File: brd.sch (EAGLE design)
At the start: 15 parts, among them IC1 OP27Z, X1 BNC-H, X2 BNC-H, X3 BNC-H, X4 BNC-H

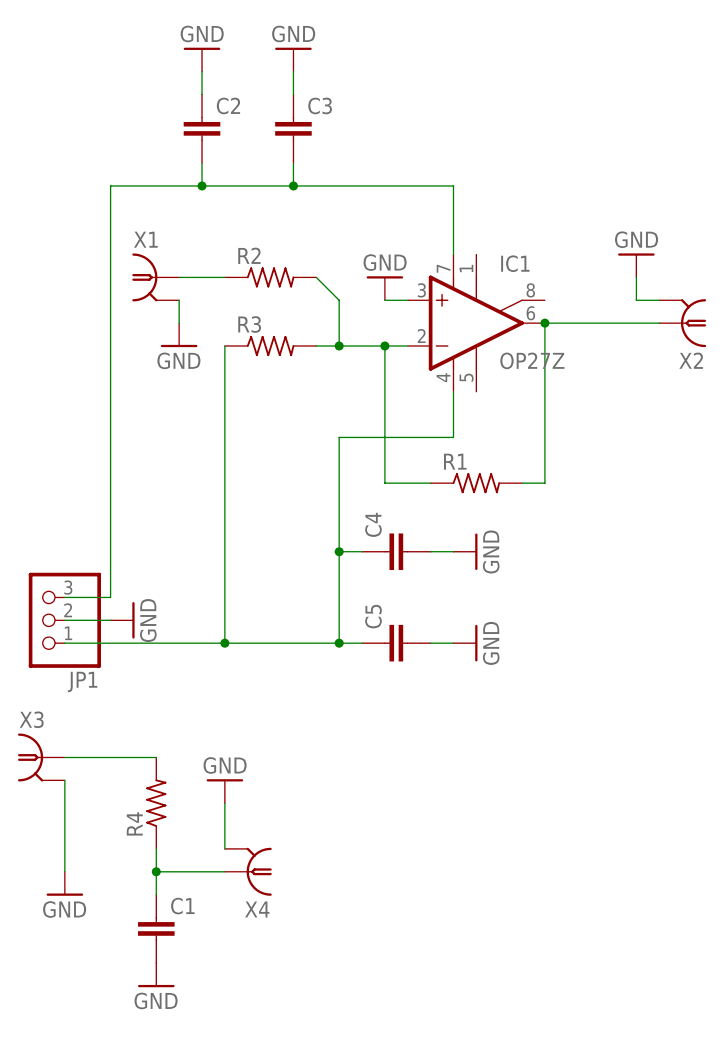
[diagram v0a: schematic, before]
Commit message: better circuit
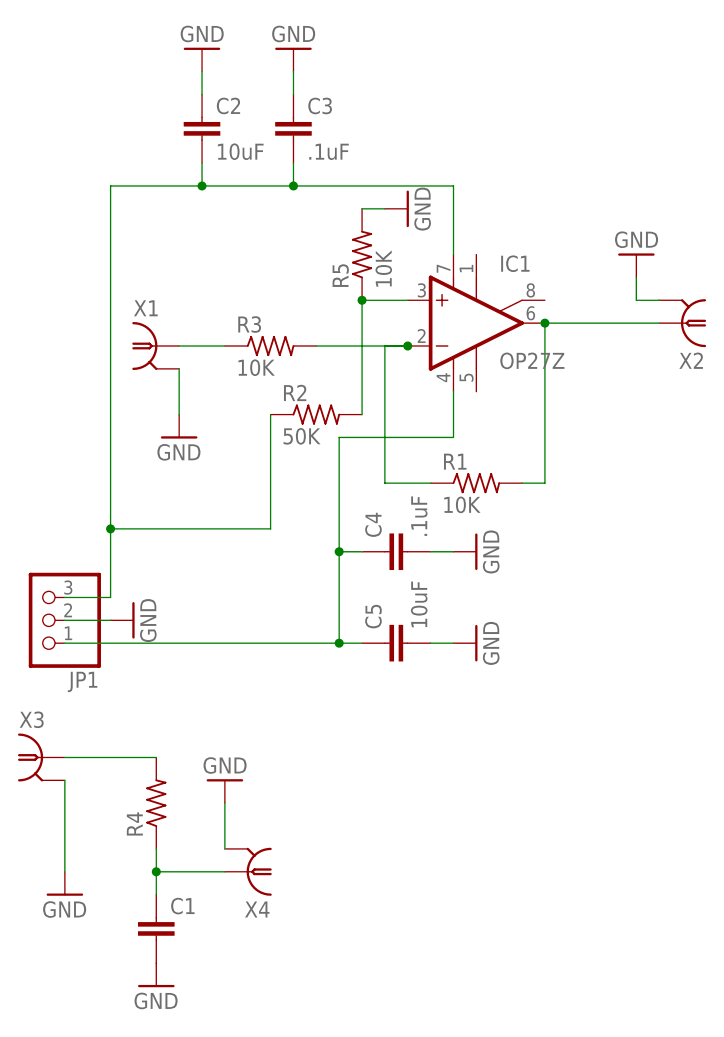
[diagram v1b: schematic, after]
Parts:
- added R5: 10K, resistor:R-US_0204/2V
- C2, C5: value (none) -> 10uF
- C3, C4: value (none) -> .1uF
- R1, R3: value (none) -> 10K
- R2: value (none) -> 50K
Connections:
- new net N$9: IC1.+IN, R2.2, R5.1
- net GND: now also R5.2; no longer IC1.+IN
- net N$1: no longer R2.2
- net N$3: no longer R3.1
- net N$6: now also R3.1; no longer R2.1
- net N$7: now also R2.1
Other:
- moved on the sheet: R2, X1
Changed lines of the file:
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@@
 <?xml version="1.0" encoding="utf-8"?>
 <!DOCTYPE eagle SYSTEM "eagle.dtd">
-<eagle version="7.5.0">
+<eagle version="8.1.0">
 <drawing>
 <settings>
@@
 <part name="GND2" library="supply1" deviceset="GND" device=""/>
 <part name="GND3" library="supply1" deviceset="GND" device=""/>
-<part name="R1" library="resistor" deviceset="R-US_" device="0204/2V"/>
-<part name="R2" library="resistor" deviceset="R-US_" device="0204/2V"/>
-<part name="R3" library="resistor" deviceset="R-US_" device="0204/2V"/>
+<part name="R1" library="resistor" deviceset="R-US_" device="0204/2V" value="10K"/>
+<part name="R2" library="resistor" deviceset="R-US_" device="0204/2V" value="50K"/>
+<part name="R3" library="resistor" deviceset="R-US_" device="0204/2V" value="10K"/>
 <part name="GND4" library="supply1" deviceset="GND" device=""/>
 <part name="GND5" library="supply1" deviceset="GND" device=""/>
@@
 <part name="R4" library="resistor" deviceset="R-US_" device="0204/2V"/>
 <part name="C1" library="resistor" deviceset="C-EU" device="025-024X044"/>
-<part name="C2" library="resistor" deviceset="C-EU" device="025-024X044"/>
-<part name="C3" library="resistor" deviceset="C-EU" device="025-024X044"/>
-<part name="C4" library="resistor" deviceset="C-EU" device="025-024X044"/>
-<part name="C5" library="resistor" deviceset="C-EU" device="025-024X044"/>
+<part name="C2" library="resistor" deviceset="C-EU" device="025-024X044" value="10uF"/>
+<part name="C3" library="resistor" deviceset="C-EU" device="025-024X044" value=".1uF"/>
+<part name="C4" library="resistor" deviceset="C-EU" device="025-024X044" value=".1uF"/>
+<part name="C5" library="resistor" deviceset="C-EU" device="025-024X044" value="10uF"/>
 <part name="GND7" library="supply1" deviceset="GND" device=""/>
 <part name="GND8" library="supply1" deviceset="GND" device=""/>
@@
 <part name="GND10" library="supply1" deviceset="GND" device=""/>
 <part name="GND11" library="supply1" deviceset="GND" device=""/>
+<part name="R5" library="resistor" deviceset="R-US_" device="0204/2V" value="10K"/>
 </parts>
 <sheets>
@@
 <instances>
 <instance part="IC1" gate="A" x="15.24" y="106.68"/>
-<instance part="GND1" gate="1" x="5.08" y="111.76" rot="R180"/>
-<instance part="X1" gate="G$1" x="-20.32" y="111.76"/>
+<instance part="GND1" gate="1" x="7.62" y="119.38" rot="R90"/>
+<instance part="X1" gate="G$1" x="-20.32" y="104.14"/>
 <instance part="X2" gate="G$1" x="38.1" y="106.68" rot="R180"/>
 <instance part="X3" gate="G$1" x="-33.02" y="58.42"/>
@@
 <instance part="JP1" gate="A" x="-33.02" y="73.66" rot="R180"/>
 <instance part="GND2" gate="1" x="-22.86" y="73.66" rot="R90"/>
-<instance part="GND3" gate="1" x="-17.78" y="104.14"/>
+<instance part="GND3" gate="1" x="-17.78" y="93.98"/>
 <instance part="R1" gate="G$1" x="15.24" y="88.9"/>
-<instance part="R2" gate="G$1" x="-7.62" y="111.76"/>
+<instance part="R2" gate="G$1" x="-2.54" y="96.52"/>
 <instance part="R3" gate="G$1" x="-7.62" y="104.14"/>
 <instance part="GND4" gate="1" x="33.02" y="114.3" rot="R180"/>
@@
 <instance part="GND10" gate="1" x="15.24" y="81.28" rot="R90"/>
 <instance part="GND11" gate="1" x="15.24" y="71.12" rot="R90"/>
+<instance part="R5" gate="G$1" x="2.54" y="114.3" rot="R90"/>
 </instances>
 <busses>
@@
 <net name="GND" class="0">
 <segment>
-<pinref part="GND1" gate="1" pin="GND"/>
-<pinref part="IC1" gate="A" pin="+IN"/>
-<wire x1="5.08" y1="109.22" x2="7.62" y2="109.22" width="0.1524" layer="91"/>
-</segment>
-<segment>
 <pinref part="X1" gate="G$1" pin="2"/>
 <pinref part="GND3" gate="1" pin="GND"/>
-<wire x1="-17.78" y1="109.22" x2="-17.78" y2="106.68" width="0.1524" layer="91"/>
+<wire x1="-17.78" y1="101.6" x2="-17.78" y2="96.52" width="0.1524" layer="91"/>
 </segment>
 <segment>
@@
 <wire x1="-30.48" y1="73.66" x2="-25.4" y2="73.66" width="0.1524" layer="91"/>
 </segment>
+<segment>
+<pinref part="R5" gate="G$1" pin="2"/>
+<pinref part="GND1" gate="1" pin="GND"/>
+<wire x1="2.54" y1="119.38" x2="5.08" y2="119.38" width="0.1524" layer="91"/>
+</segment>
 </net>
 <net name="N$1" class="0">
 <segment>
 <pinref part="IC1" gate="A" pin="-IN"/>
-<wire x1="-2.54" y1="104.14" x2="0" y2="104.14" width="0.1524" layer="91"/>
-<wire x1="0" y1="104.14" x2="5.08" y2="104.14" width="0.1524" layer="91"/>
 <wire x1="5.08" y1="104.14" x2="7.62" y2="104.14" width="0.1524" layer="91"/>
 <wire x1="5.08" y1="104.14" x2="5.08" y2="88.9" width="0.1524" layer="91"/>
-<junction x="5.08" y="104.14"/>
 <wire x1="5.08" y1="88.9" x2="10.16" y2="88.9" width="0.1524" layer="91"/>
+<pinref part="R1" gate="G$1" pin="1"/>
 <pinref part="R3" gate="G$1" pin="2"/>
-<pinref part="R1" gate="G$1" pin="1"/>
-<pinref part="R2" gate="G$1" pin="2"/>
-<wire x1="-2.54" y1="111.76" x2="0" y2="109.22" width="0.1524" layer="91"/>
-<wire x1="0" y1="109.22" x2="0" y2="104.14" width="0.1524" layer="91"/>
-<junction x="0" y="104.14"/>
+<wire x1="-2.54" y1="104.14" x2="7.62" y2="104.14" width="0.1524" layer="91"/>
+<junction x="7.62" y="104.14"/>
 </segment>
 </net>
@@
 <wire x1="12.7" y1="93.98" x2="12.7" y2="99.06" width="0.1524" layer="91"/>
 <pinref part="JP1" gate="A" pin="1"/>
-<wire x1="-30.48" y1="71.12" x2="-12.7" y2="71.12" width="0.1524" layer="91"/>
-<wire x1="-12.7" y1="71.12" x2="0" y2="71.12" width="0.1524" layer="91"/>
+<wire x1="-30.48" y1="71.12" x2="0" y2="71.12" width="0.1524" layer="91"/>
 <wire x1="0" y1="71.12" x2="0" y2="81.28" width="0.1524" layer="91"/>
 <wire x1="0" y1="81.28" x2="0" y2="93.98" width="0.1524" layer="91"/>
@@
 <wire x1="2.54" y1="71.12" x2="0" y2="71.12" width="0.1524" layer="91"/>
 <junction x="0" y="71.12"/>
-<pinref part="R3" gate="G$1" pin="1"/>
-<wire x1="-12.7" y1="104.14" x2="-12.7" y2="71.12" width="0.1524" layer="91"/>
-<junction x="-12.7" y="71.12"/>
-</segment>
-</net>
-<net name="N$6" class="0">
-<segment>
-<pinref part="X1" gate="G$1" pin="1"/>
-<wire x1="-17.78" y1="111.76" x2="-12.7" y2="111.76" width="0.1524" layer="91"/>
-<pinref part="R2" gate="G$1" pin="1"/>
 </segment>
 </net>
@@
 <wire x1="-5.08" y1="121.92" x2="12.7" y2="121.92" width="0.1524" layer="91"/>
 <wire x1="12.7" y1="121.92" x2="12.7" y2="114.3" width="0.1524" layer="91"/>
-<wire x1="-25.4" y1="76.2" x2="-25.4" y2="121.92" width="0.1524" layer="91"/>
+<wire x1="-25.4" y1="76.2" x2="-25.4" y2="83.82" width="0.1524" layer="91"/>
 <pinref part="C2" gate="G$1" pin="2"/>
+<wire x1="-25.4" y1="83.82" x2="-25.4" y2="121.92" width="0.1524" layer="91"/>
 <wire x1="-15.24" y1="124.46" x2="-15.24" y2="121.92" width="0.1524" layer="91"/>
 <junction x="-15.24" y="121.92"/>
@@
 <wire x1="-5.08" y1="124.46" x2="-5.08" y2="121.92" width="0.1524" layer="91"/>
 <junction x="-5.08" y="121.92"/>
+<wire x1="-25.4" y1="83.82" x2="-7.62" y2="83.82" width="0.1524" layer="91"/>
+<junction x="-25.4" y="83.82"/>
+<pinref part="R2" gate="G$1" pin="1"/>
+<wire x1="-7.62" y1="83.82" x2="-7.62" y2="96.52" width="0.1524" layer="91"/>
 </segment>
 </net>
@@
 </segment>
 </net>
+<net name="N$9" class="0">
+<segment>
+<pinref part="IC1" gate="A" pin="+IN"/>
+<wire x1="2.54" y1="109.22" x2="7.62" y2="109.22" width="0.1524" layer="91"/>
+<pinref part="R5" gate="G$1" pin="1"/>
+<pinref part="R2" gate="G$1" pin="2"/>
+<wire x1="2.54" y1="96.52" x2="2.54" y2="109.22" width="0.1524" layer="91"/>
+<junction x="2.54" y="109.22"/>
+</segment>
+</net>
+<net name="N$6" class="0">
+<segment>
+<pinref part="X1" gate="G$1" pin="1"/>
+<pinref part="R3" gate="G$1" pin="1"/>
+<wire x1="-17.78" y1="104.14" x2="-12.7" y2="104.14" width="0.1524" layer="91"/>
+</segment>
+</net>
